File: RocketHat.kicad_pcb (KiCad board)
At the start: 2 copper layers, 72.2 x 58.1 mm, 28 parts, among them J1 Conn_01x06_Female, J10 Conn_01x10_Female, J11 Raspberry_Pi_2_3, J2 Conn_01x06_Female, J3 Conn_01x07_Female, J4 Conn_01x06_Female, J5 Conn_01x04_Female, J6 Conn_01x02_Female, J7 Conn_01x02, J8 Conn_01x10_Female, J9 Conn_01x02, Q1 2N3904, Q2 DMG2305UX-13, Q3 2N3904, U1 CAT24C128

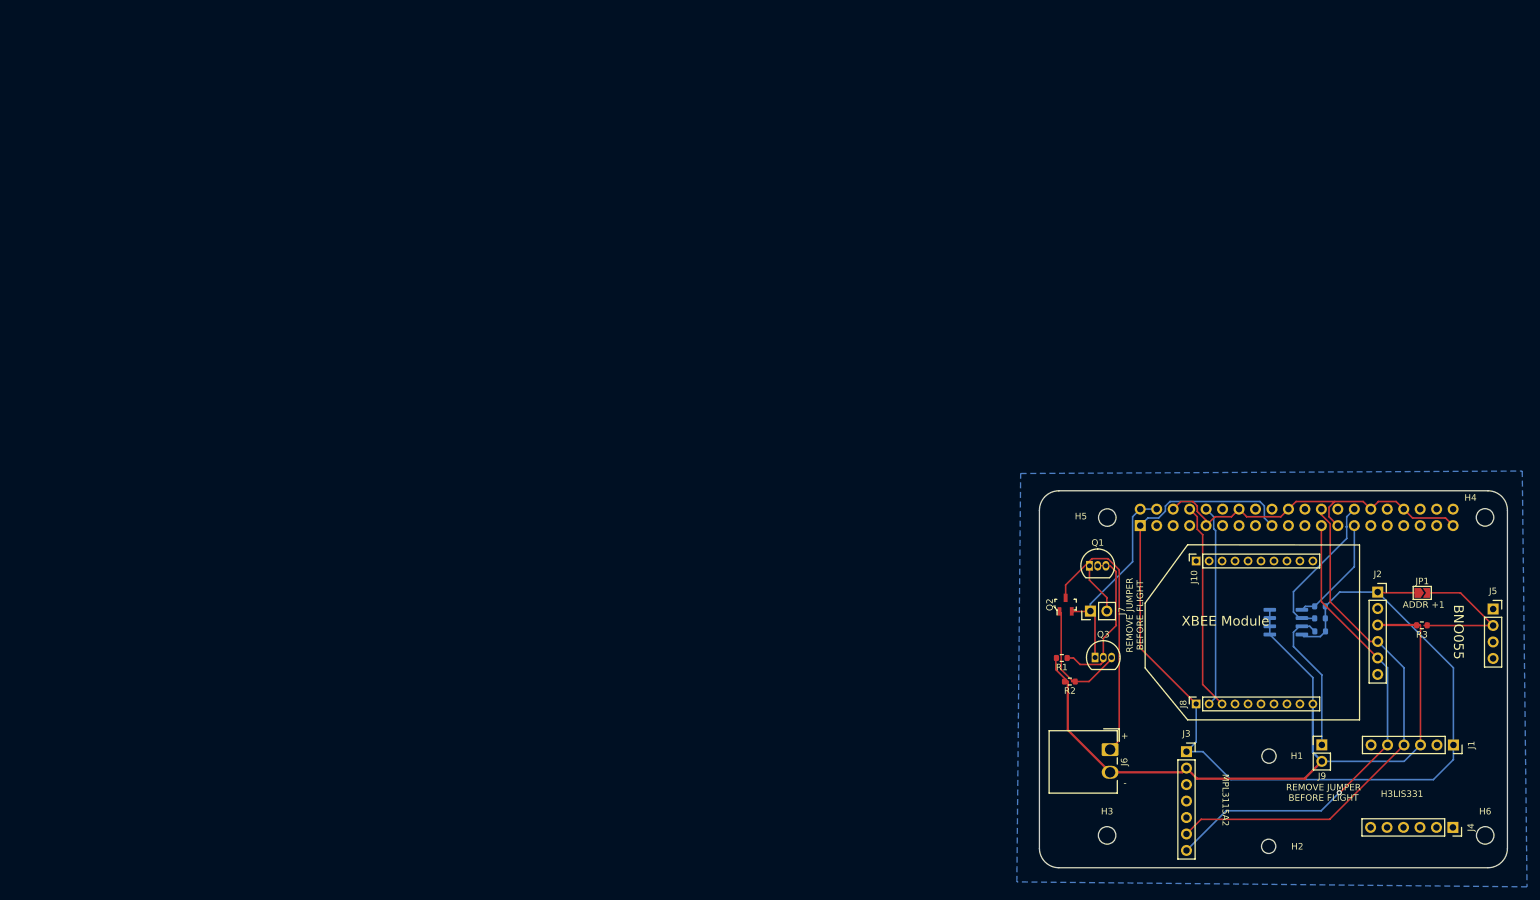
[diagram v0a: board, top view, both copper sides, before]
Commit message: Smol Board
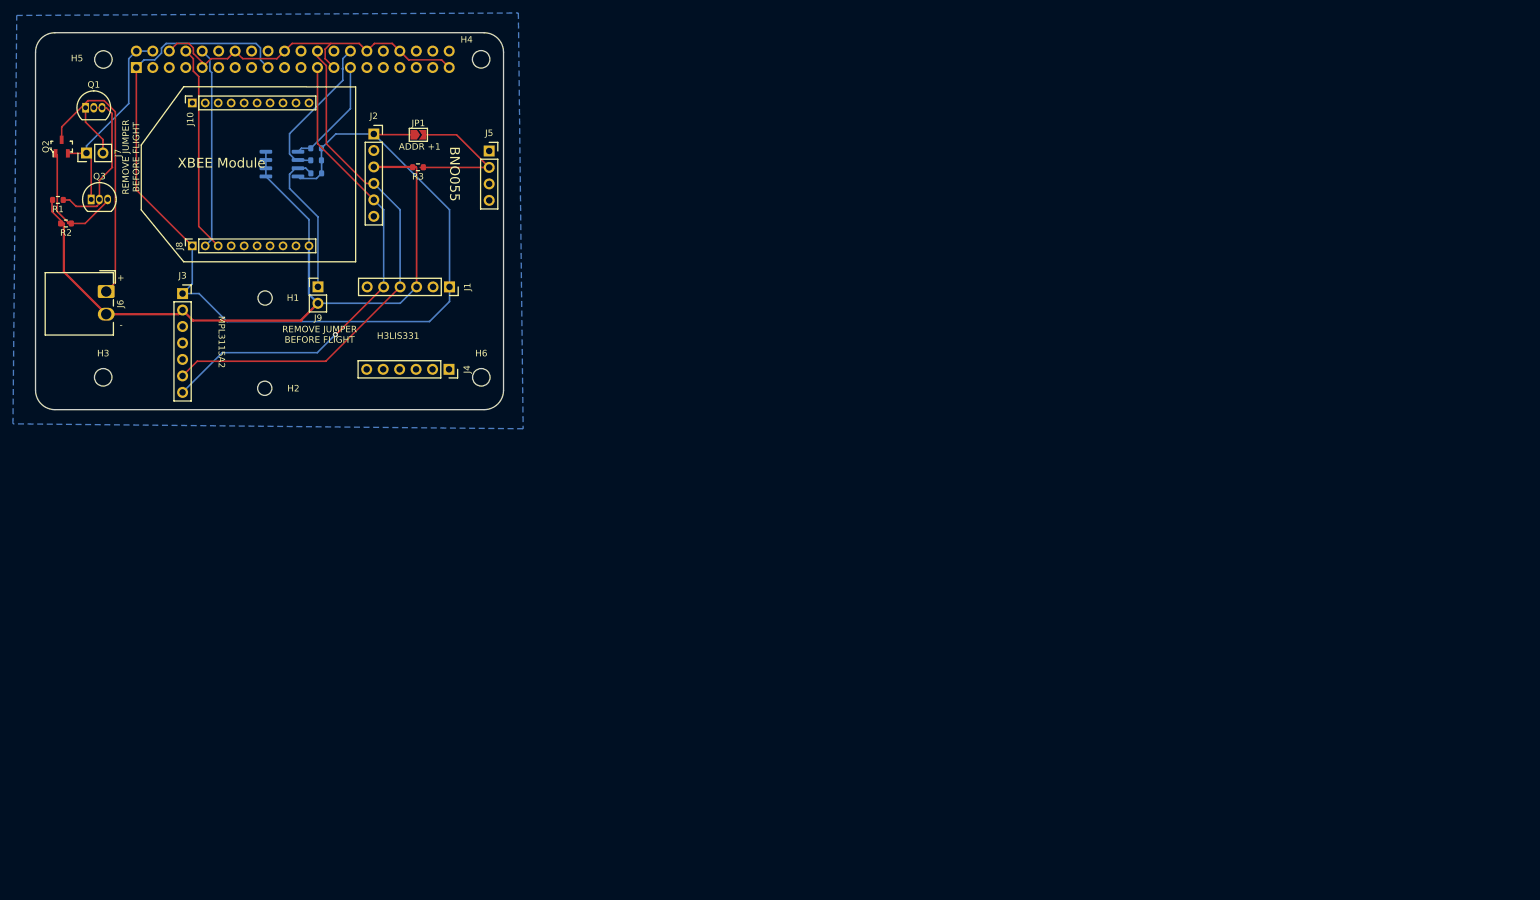
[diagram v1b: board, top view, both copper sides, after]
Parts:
- moved H2 170.2 mm to (77.5, 78.0)
- moved H3 170.2 mm to (52.5, 76.4)
- moved H4 170.2 mm to (110.8, 27.3)
- moved H6 170.2 mm to (110.9, 76.4)
- moved J1 170.2 mm to (106.0, 62.4)
- moved J10 170.2 mm to (66.3, 34.0)
- moved J5 170.2 mm to (112.1, 41.4)
- moved J8 170.2 mm to (66.3, 56.1)
- moved JP1 170.2 mm to (101.2, 38.9)
- moved Q2 170.2 mm to (46.1, 40.8)
- moved R1 170.2 mm to (45.6, 49.0)
- moved R3 170.2 mm to (101.1, 43.9)
- moved H1 170.2 mm to (77.5, 64.1)
- moved H5 170.2 mm to (52.6, 27.3)
- moved J11 170.2 mm to (57.7, 28.6)
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
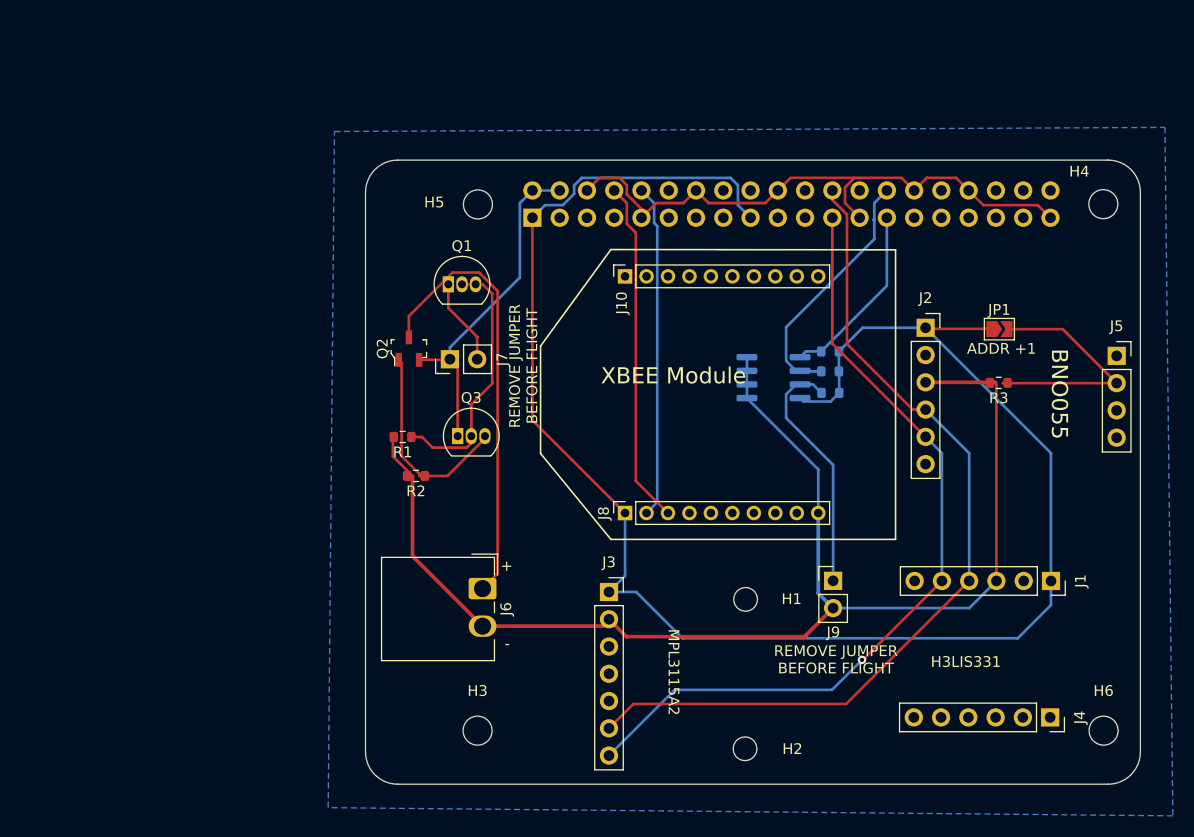
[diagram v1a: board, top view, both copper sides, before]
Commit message: Even SMOLLER Board
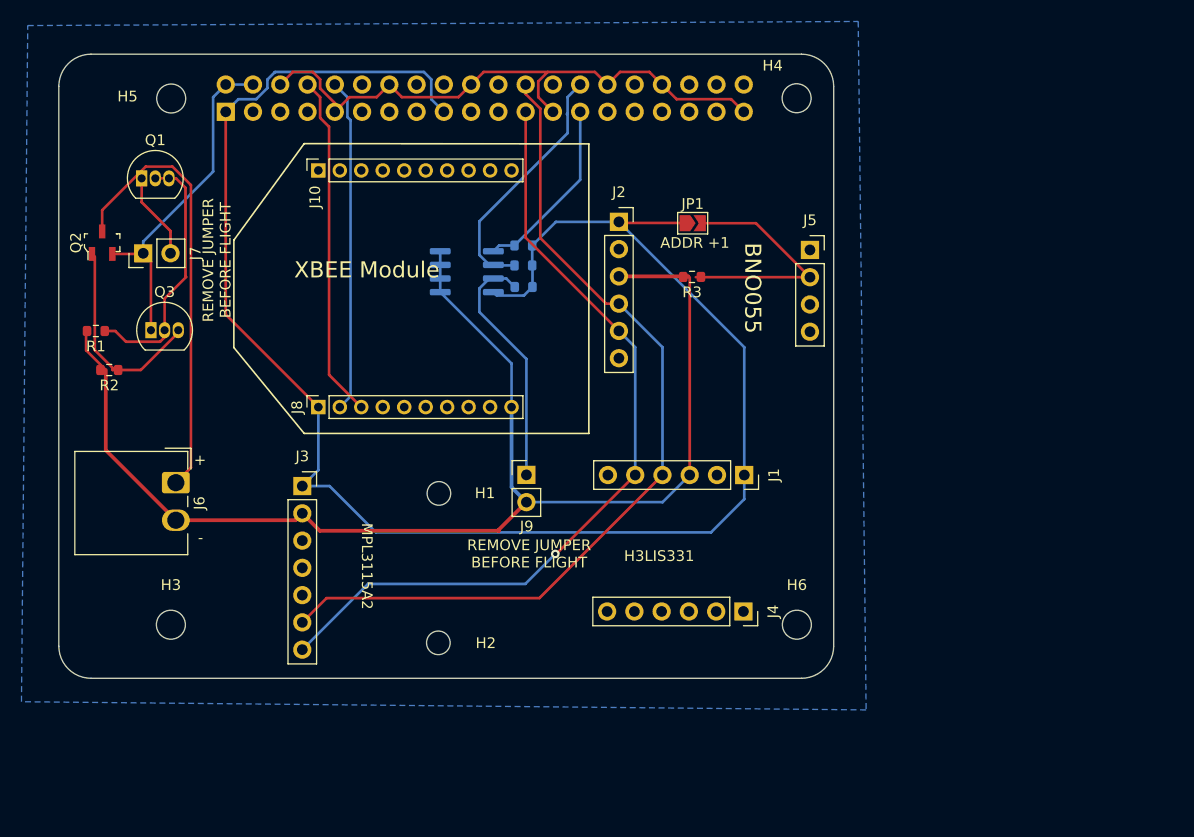
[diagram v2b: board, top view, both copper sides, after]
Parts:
- moved H1 30.2 mm to (48.9, 54.3)
- moved R5 30.2 mm to (56.8, 31.2)
- moved R6 30.2 mm to (56.8, 33.0)
- moved H4 30.2 mm to (82.3, 17.4)
- moved H5 30.2 mm to (24.0, 17.5)
- moved J1 30.2 mm to (77.4, 52.5)
- moved J10 30.2 mm to (37.7, 24.2)
- moved J11 30.2 mm to (29.1, 18.7)
- moved J2 30.2 mm to (65.7, 29.0)
- moved J5 30.2 mm to (83.5, 31.6)
- moved J7 30.2 mm to (21.4, 31.9)
- moved Q1 30.2 mm to (21.3, 24.9)
- moved Q2 30.2 mm to (17.6, 30.9)
- moved R2 30.2 mm to (18.2, 42.8)
- moved J6 30.2 mm to (24.4, 53.2)
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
